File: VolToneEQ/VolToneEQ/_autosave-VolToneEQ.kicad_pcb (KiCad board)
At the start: 4 copper layers, 149.4 x 87.7 mm, 91 parts, among them Q1 ZTX951, Q2 ZTX951, U1 TL072, U2 TL072, U3 TL072, U4 TL072

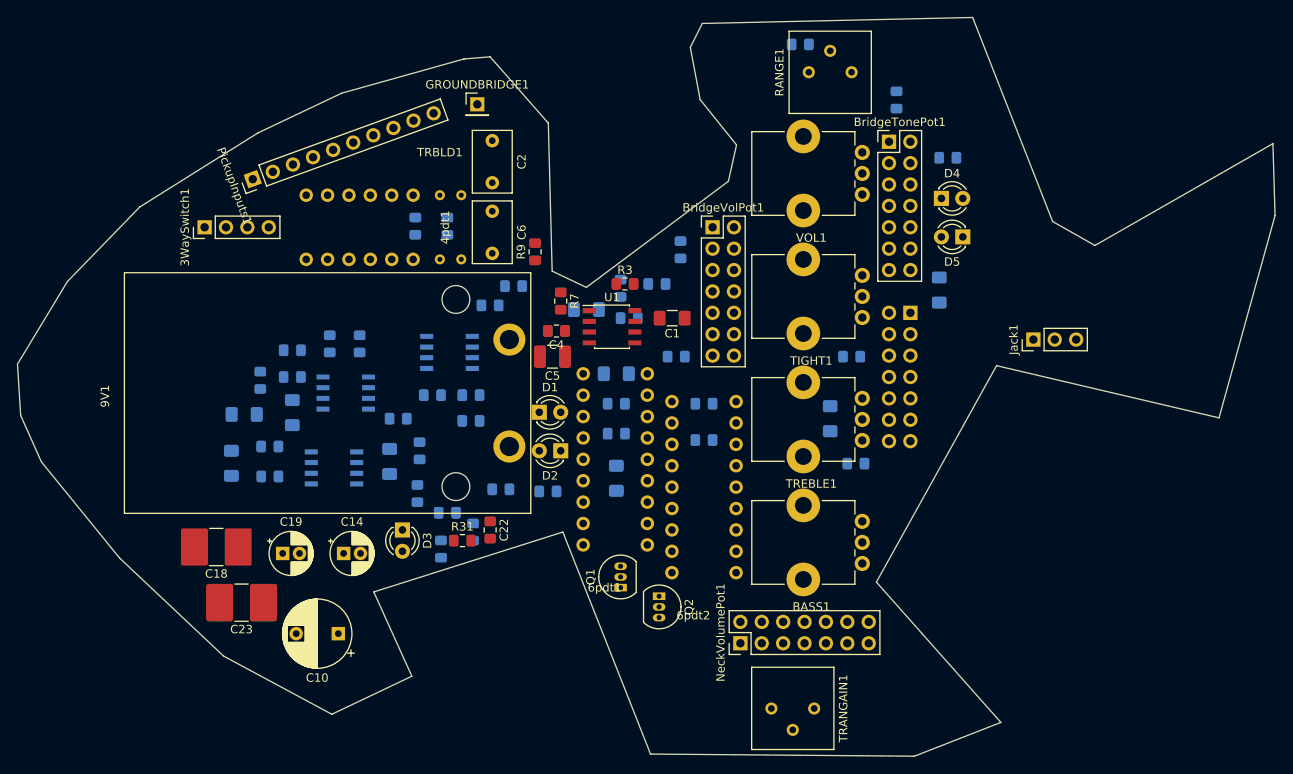
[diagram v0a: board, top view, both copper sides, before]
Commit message: routed board
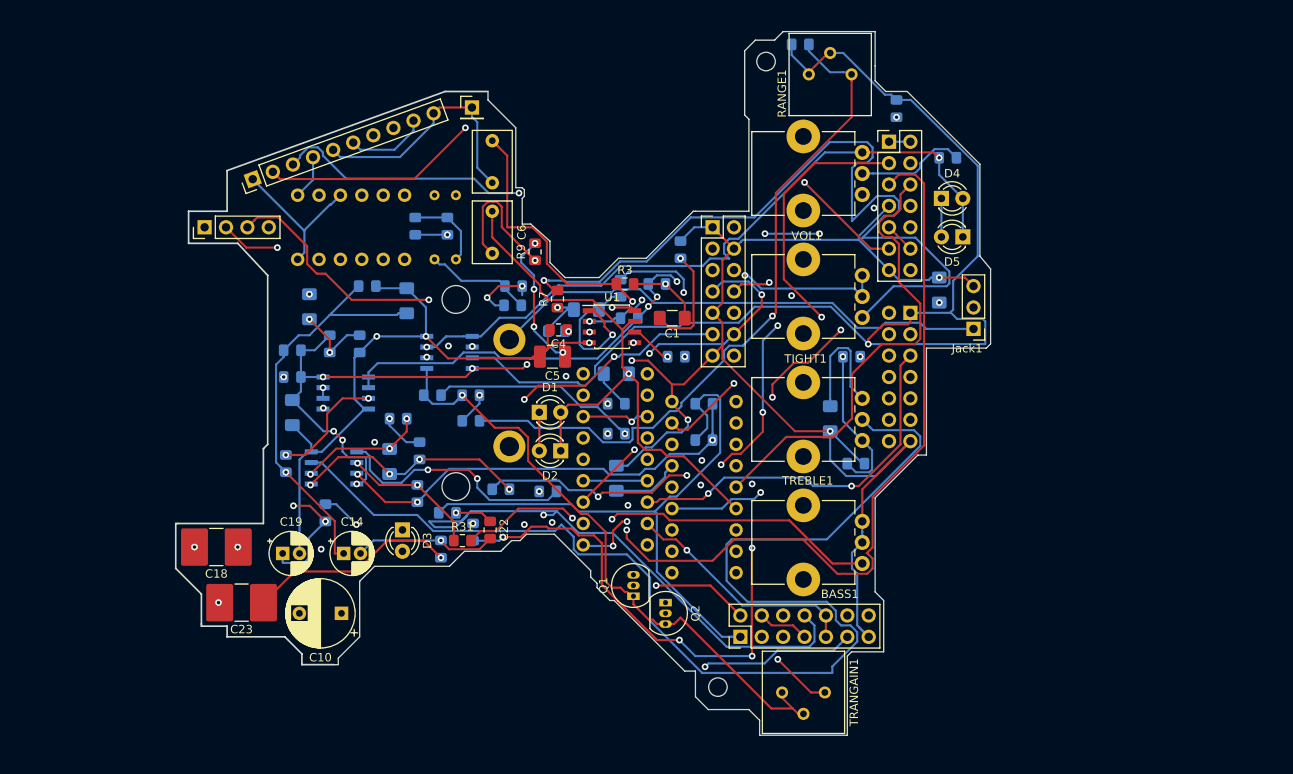
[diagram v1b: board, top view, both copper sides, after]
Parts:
- added REF**: MountingHole_2.2mm_M2, Mounting_Holes:MountingHole_2.2mm_M2, F.Cu at (114.3, 109.2)
- added REF**: MountingHole_2.2mm_M2, Mounting_Holes:MountingHole_2.2mm_M2, F.Cu at (108.6, 183.5)
- moved C15 23.6 mm to (71.6, 137.6), turned to 90 degrees
- moved C20 20.8 mm to (60.1, 138.3)
- moved R21 16.9 mm to (66.9, 135.9), turned to 0 degrees
- moved R28 7.89 mm to (62.0, 162.8), turned to 270 degrees
- moved Jack1 7.22 mm to (138.9, 141.0), turned to 180 degrees
- moved R22 2.79 mm to (57.3, 157.0), turned to 270 degrees
- moved C26 2.68 mm to (84.2, 138.2)
- moved C10 2.44 mm to (63.9, 174.8)
- moved TRANGAIN1 2.29 mm to (116.2, 184.2)
- moved Q1 1.83 mm to (98.6, 172.7)
- moved Q2 1.08 mm to (102.4, 173.5)
- moved R35 1.03 mm to (129.8, 114.8)
- moved 4pdt1 1.02 mm to (84.1, 130.2)
- moved NeckVolumePot1 0.76 mm to (111.3, 177.5)
- moved GROUNDBRIDGE1 0.74 mm to (79.4, 114.7)
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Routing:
- net BRGRN2: track 0.00 -> 345.3 mm, vias 0 -> 9
- net OUT: track 0.00 -> 154.9 mm, vias 0 -> 1
- net Net-(TREBLE1-Pad2): track 0.00 -> 142.5 mm
- net PRESIN: track 0.00 -> 137.8 mm, vias 0 -> 1
- net NBLACK: track 0.00 -> 124.4 mm
- net NOUT: track 0.00 -> 118.7 mm, vias 0 -> 2
- net NRED2: track 0.00 -> 102.7 mm, vias 0 -> 1
- net ODMIDIN: track 0.00 -> 102.2 mm, vias 0 -> 4
- net BRBLACK: track 0.00 -> 101.7 mm, vias 0 -> 2
- net BRRED2: track 0.00 -> 101.5 mm, vias 0 -> 3
- net Vref2: track 0.00 -> 98.8 mm, vias 0 -> 3
- net Net-(R7-Pad2): track 0.00 -> 98.0 mm, vias 0 -> 1
- net NGRN2: track 0.00 -> 94.4 mm, vias 0 -> 2
- net BTONEIN: track 0.00 -> 93.7 mm, vias 0 -> 1
- net BRWHT: track 0.00 -> 91.0 mm, vias 0 -> 2
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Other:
- board size 149.4 x 87.7 mm -> 96.8 x 83.6 mm
- rule via_min_size: 0.6858 -> 0.508
